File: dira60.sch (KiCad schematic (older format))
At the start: 21 parts, among them U0 ATmega32U4-AU, X0 XTAL_GND

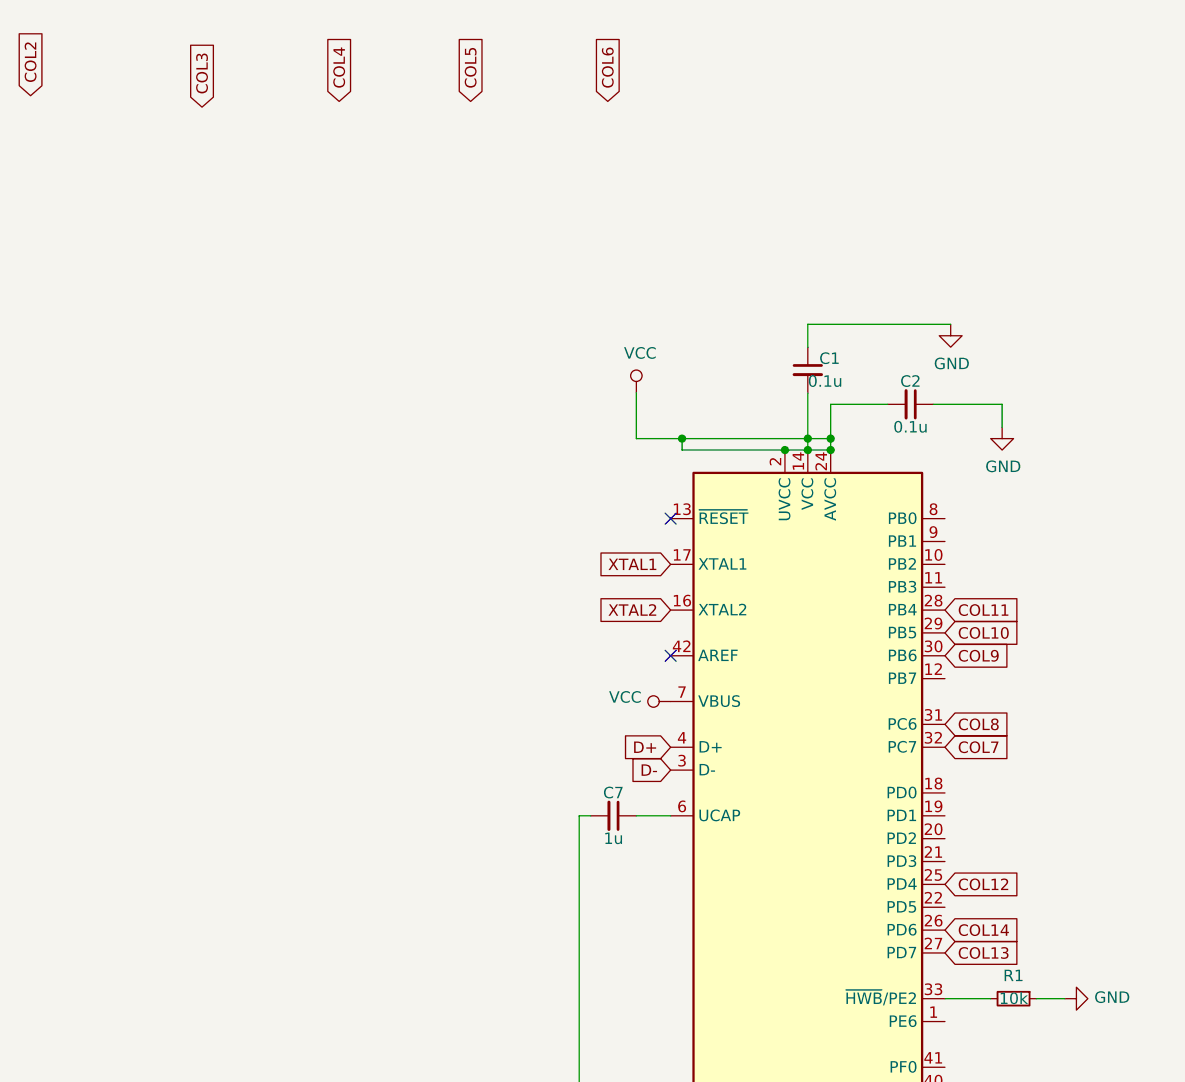
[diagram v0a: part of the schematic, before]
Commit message: Routed all cols
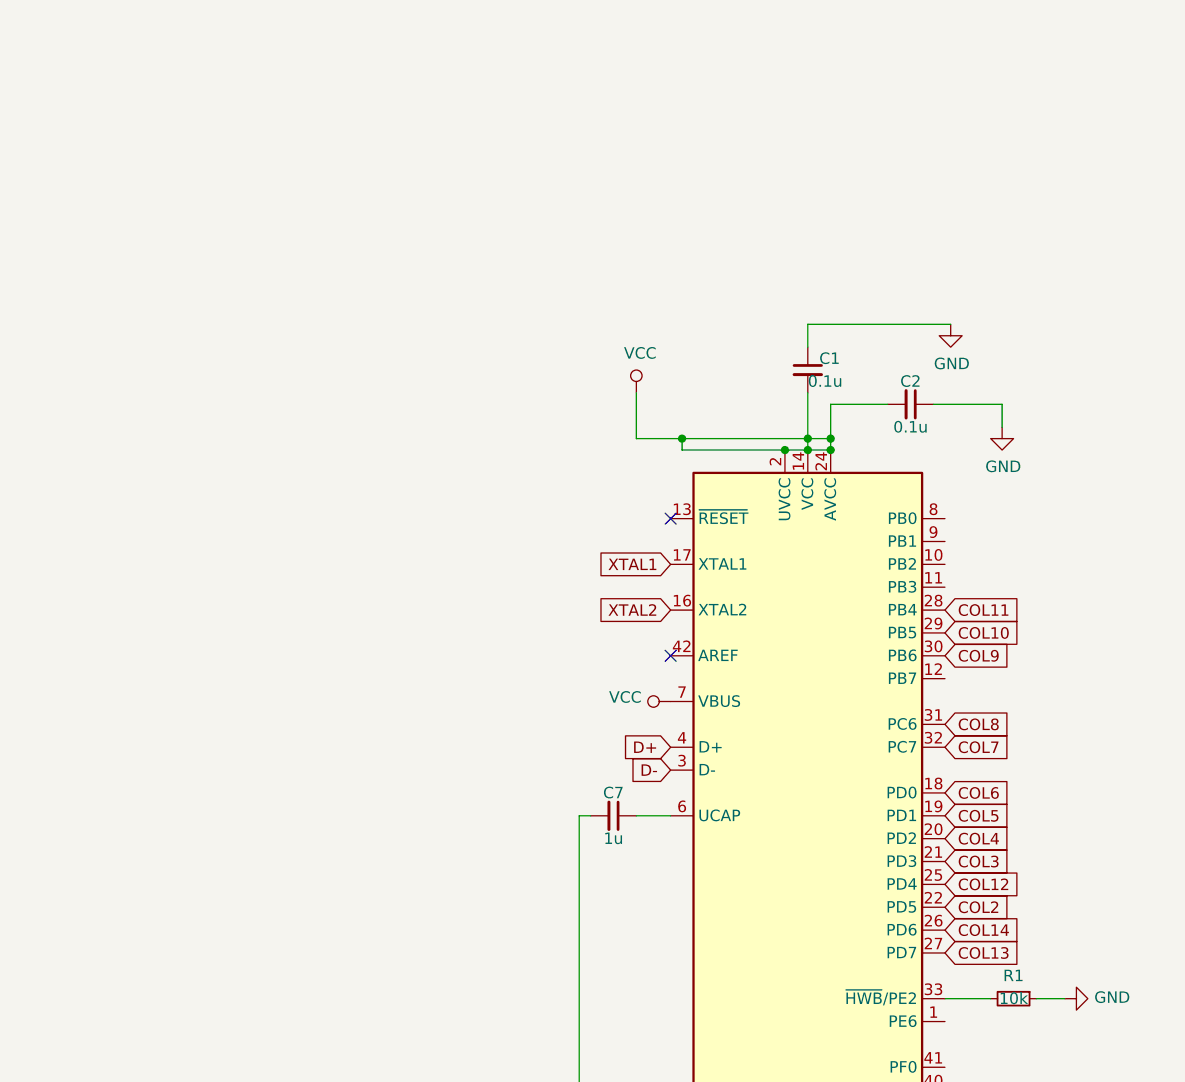
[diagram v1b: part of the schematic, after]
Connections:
- net COL2: now also U0.22 (PD5)
- net COL3: now also U0.21 (PD3)
- net COL4: now also U0.20 (PD2)
- net COL5: now also U0.19 (PD1)
- net COL6: now also U0.18 (PD0)
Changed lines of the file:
@@
 Text GLabel 6100 2750 2    50   Input ~ 0
 COL7
-Text GLabel 4625 -75  1    50   Input ~ 0
+Text GLabel 6100 2950 2    50   Input ~ 0
 COL6
-Text GLabel 4025 -75  1    50   Input ~ 0
+Text GLabel 6100 3050 2    50   Input ~ 0
 COL5
-Text GLabel 3450 -75  1    50   Input ~ 0
+Text GLabel 6100 3150 2    50   Input ~ 0
 COL4
-Text GLabel 2850 -50  1    50   Input ~ 0
+Text GLabel 6100 3250 2    50   Input ~ 0
 COL3
-Text GLabel 2100 -100 1    50   Input ~ 0
+Text GLabel 6100 3450 2    50   Input ~ 0
 COL2
 Text GLabel 7150 3700 2    50   Input ~ 0
